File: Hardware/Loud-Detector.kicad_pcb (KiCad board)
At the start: 2 copper layers, 59.7 x 47.6 mm, 27 parts, among them J1 TP4056, J2 ON_OFF, J3 VIN+, J4 VIN-, J5 VOUT+, J6 VOUT-, J7 KY-037, J8 BUZZER, Q1 BC557, Q2 BC547, U1 ATtiny85, U2 MT3608_Module

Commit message: PCB minor improvements
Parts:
- RV1: value 10K -> 5K
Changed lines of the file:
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@@
 			)
 		)
-		(property "Value" "10K"
+		(property "Value" "5K"
 			(at 5 0.525 90)
 			(layer "F.Fab")
@@
 	)
 	(zone
-		(net 12)
-		(net_name "Net-(R1-Pad1)")
+		(net 19)
+		(net_name "Net-(J8-Pin_1)")
 		(layer "B.Cu")
 		(name "$teardrop_padvia$")
 		(hatch none 0.1)
-		(priority 30000)
+		(priority 30001)
 		(attr
 			(teardrop
@@
 		(polygon
 			(pts
-				(xy 130.694 91.941) (xy 128.894 91.941) (xy 128.794 92.941) (xy 129.794 94.442) (xy 130.794 92.941)
+				(xy 177.049 91.861) (xy 175.249 91.861) (xy 175.149 92.861) (xy 176.149 94.362) (xy 177.149 92.861)
 			)
 		)
 	)
 	(zone
-		(net 19)
-		(net_name "Net-(J8-Pin_1)")
+		(net 2)
+		(net_name "+5V")
 		(layer "B.Cu")
 		(name "$teardrop_padvia$")
@@
 		(polygon
 			(pts
-				(xy 177.049 91.861) (xy 175.249 91.861) (xy 175.149 92.861) (xy 176.149 94.362) (xy 177.149 92.861)
+				(xy 128.379408 102.763383) (xy 127.106617 101.490592) (xy 126.566162 102.941) (xy 127.293293 104.441707)
+				(xy 128.601343 102.952406)
 			)
 		)
 	)
 	(zone
-		(net 1)
-		(net_name "GND")
+		(net 12)
+		(net_name "Net-(R1-Pad1)")
 		(layer "B.Cu")
-		(name "GND")
-		(hatch edge 0.5)
+		(name "$teardrop_padvia$")
+		(hatch none 0.1)
+		(priority 30000)
+		(attr
+			(teardrop
+				(type padvia)
+			)
+		)
 		(connect_pads yes
-			(clearance 1)
+			(clearance 0)
 		)
-		(min_thickness 0.25)
+		(min_thickness 0.0254)
 		(filled_areas_thickness no)
 		(fill yes
 			(thermal_gap 0.5)
 			(thermal_bridge_width 0.5)
+			(island_removal_mode 1)
+			(island_area_min 10)
 		)
 		(polygon
 			(pts
-				(xy 122.809 60.071) (xy 122.809 107.696) (xy 182.499 107.696) (xy 182.499 60.071)
+				(xy 130.694 91.941) (xy 128.894 91.941) (xy 128.794 92.941) (xy 129.794 94.442) (xy 130.794 92.941)
 			)
 		)
 	)
 	(zone
-		(net 2)
-		(net_name "+5V")
+		(net 1)
+		(net_name "GND")
 		(layer "B.Cu")
-		(name "$teardrop_padvia$")
-		(hatch none 0.1)
-		(priority 30002)
-		(attr
-			(teardrop
-				(type padvia)
-			)
-		)
+		(name "GND")
+		(hatch edge 0.5)
 		(connect_pads yes
-			(clearance 0)
+			(clearance 1)
 		)
-		(min_thickness 0.0254)
+		(min_thickness 0.25)
 		(filled_areas_thickness no)
 		(fill yes
 			(thermal_gap 0.5)
 			(thermal_bridge_width 0.5)
-			(island_removal_mode 1)
-			(island_area_min 10)
 		)
 		(polygon
 			(pts
-				(xy 128.379408 102.763383) (xy 127.106617 101.490592) (xy 126.566162 102.941) (xy 127.293293 104.441707)
-				(xy 128.601343 102.952406)
+				(xy 122.809 60.071) (xy 122.809 107.696) (xy 182.499 107.696) (xy 182.499 60.071)
 			)
 		)

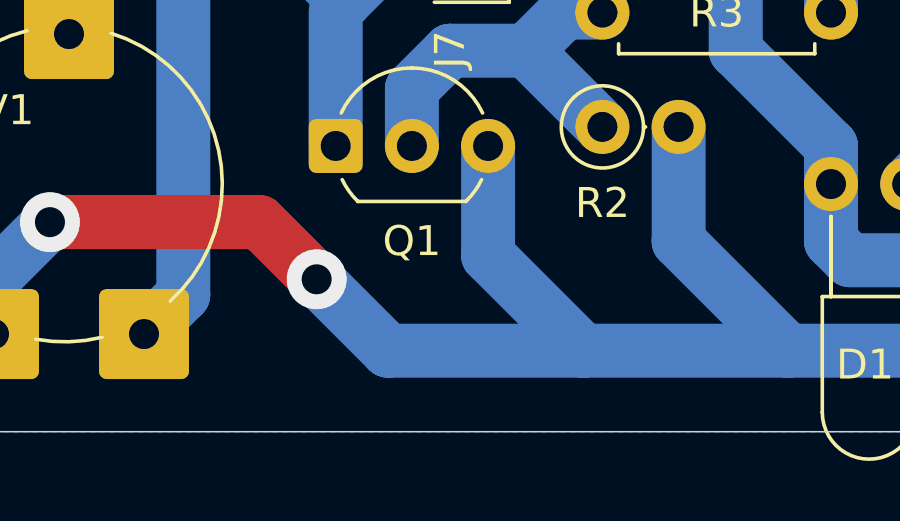
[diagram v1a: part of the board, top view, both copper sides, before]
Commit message: PCB minor improvements
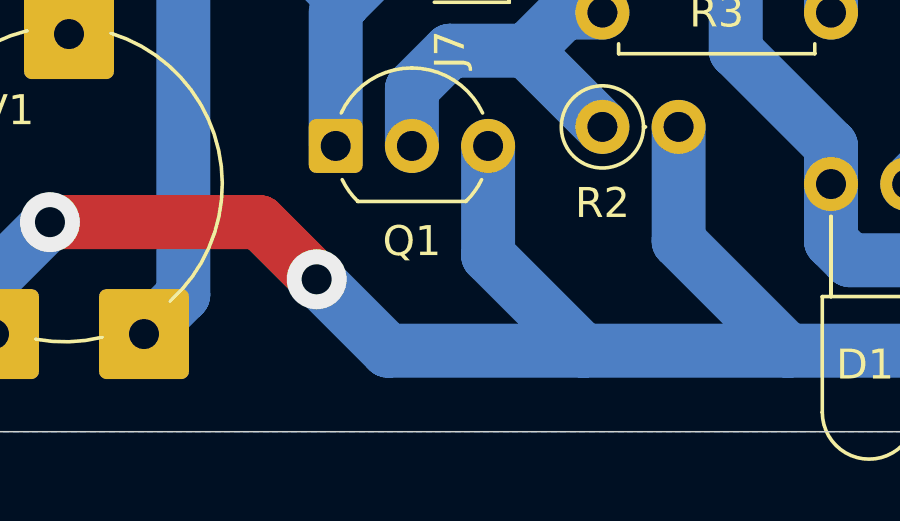
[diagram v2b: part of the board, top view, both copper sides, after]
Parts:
- RV1: value 5K -> 10K
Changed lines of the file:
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@@
 			)
 		)
-		(property "Value" "5K"
+		(property "Value" "10K"
 			(at 5 0.525 90)
 			(layer "F.Fab")
@@
 	)
 	(segment
+		(start 140.429 104.996)
+		(end 138.049 102.616)
+		(width 1.8)
+		(layer "B.Cu")
+		(net 2)
+	)
+	(segment
 		(start 172.339 99.441)
 		(end 178.054 99.441)
@@
 	)
 	(segment
-		(start 140.429 104.996)
-		(end 146.939 104.996)
-		(width 1.8)
-		(layer "B.Cu")
-		(net 2)
-	)
-	(segment
-		(start 138.049 102.616)
+		(start 146.939 104.996)
 		(end 140.429 104.996)
 		(width 1.8)
@@
 	)
 	(segment
+		(start 146.939 104.996)
+		(end 146.845 104.902)
+		(width 1.8)
+		(layer "B.Cu")
+		(net 2)
+	)
+	(segment
 		(start 180.594 96.901)
 		(end 178.649 98.846)
@@
 	)
 	(zone
-		(net 19)
-		(net_name "Net-(J8-Pin_1)")
+		(net 2)
+		(net_name "+5V")
 		(layer "B.Cu")
 		(name "$teardrop_padvia$")
@@
 		(polygon
 			(pts
-				(xy 177.049 91.861) (xy 175.249 91.861) (xy 175.149 92.861) (xy 176.149 94.362) (xy 177.149 92.861)
+				(xy 128.379408 102.763383) (xy 127.106617 101.490592) (xy 126.566162 102.941) (xy 127.293293 104.441707)
+				(xy 128.601343 102.952406)
 			)
 		)
 	)
 	(zone
-		(net 2)
-		(net_name "+5V")
+		(net 19)
+		(net_name "Net-(J8-Pin_1)")
 		(layer "B.Cu")
 		(name "$teardrop_padvia$")
@@
 		(polygon
 			(pts
-				(xy 128.379408 102.763383) (xy 127.106617 101.490592) (xy 126.566162 102.941) (xy 127.293293 104.441707)
-				(xy 128.601343 102.952406)
+				(xy 177.049 91.861) (xy 175.249 91.861) (xy 175.149 92.861) (xy 176.149 94.362) (xy 177.149 92.861)
 			)
 		)
@@
 			)
 		)
+	)
+	(zone
+		(net 12)
+		(net_name "Net-(R1-Pad1)")
+		(layer "B.Cu")
+		(name "$teardrop_padvia$")
+		(hatch none 0.1)
+		(priority 30002)
+		(attr
+			(teardrop
+				(type padvia)
+			)
+		)
+		(connect_pads yes
+			(clearance 0)
+		)
+		(min_thickness 0.0254)
+		(filled_areas_thickness no)
+		(fill yes
+			(thermal_gap 0.5)
+			(thermal_bridge_width 0.5)
+			(island_removal_mode 1)
+			(island_area_min 10)
+		)
+		(polygon
+			(pts
+				(xy 128.379408 102.763383) (xy 127.106617 101.490592) (xy 126.566162 102.941) (xy 127.293293 104.441707)
+				(xy 128.601343 102.952406)
+			)
+		)
